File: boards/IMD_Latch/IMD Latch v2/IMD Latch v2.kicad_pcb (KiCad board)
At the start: 2 copper layers, 40 x 35 mm, 17 parts, among them J1 micromatch_female_RA_8, J2 Ultrafit_2, K1 G5Q-1A4-DC5-5V, Q1 SSM3K333R, U1 CD4043BPWR

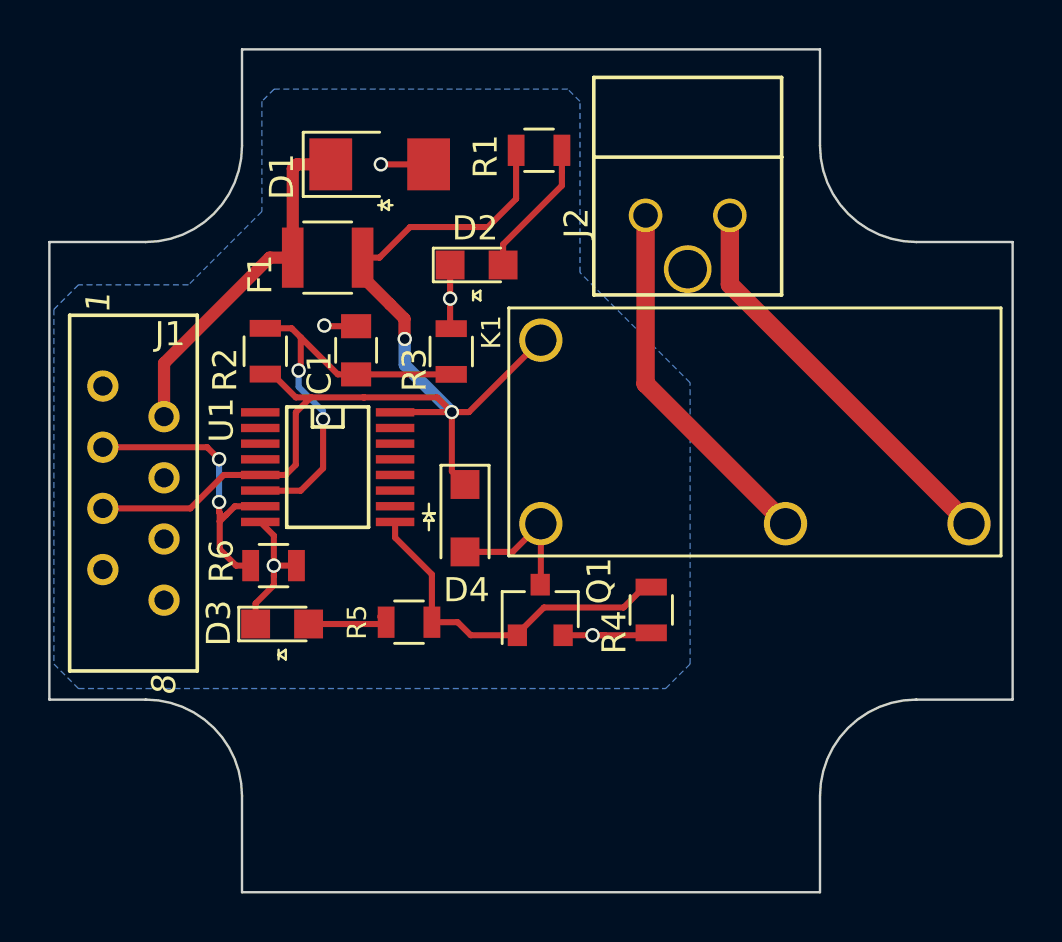
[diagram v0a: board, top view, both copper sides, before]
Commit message: IMD Latch v2 not yet checked off
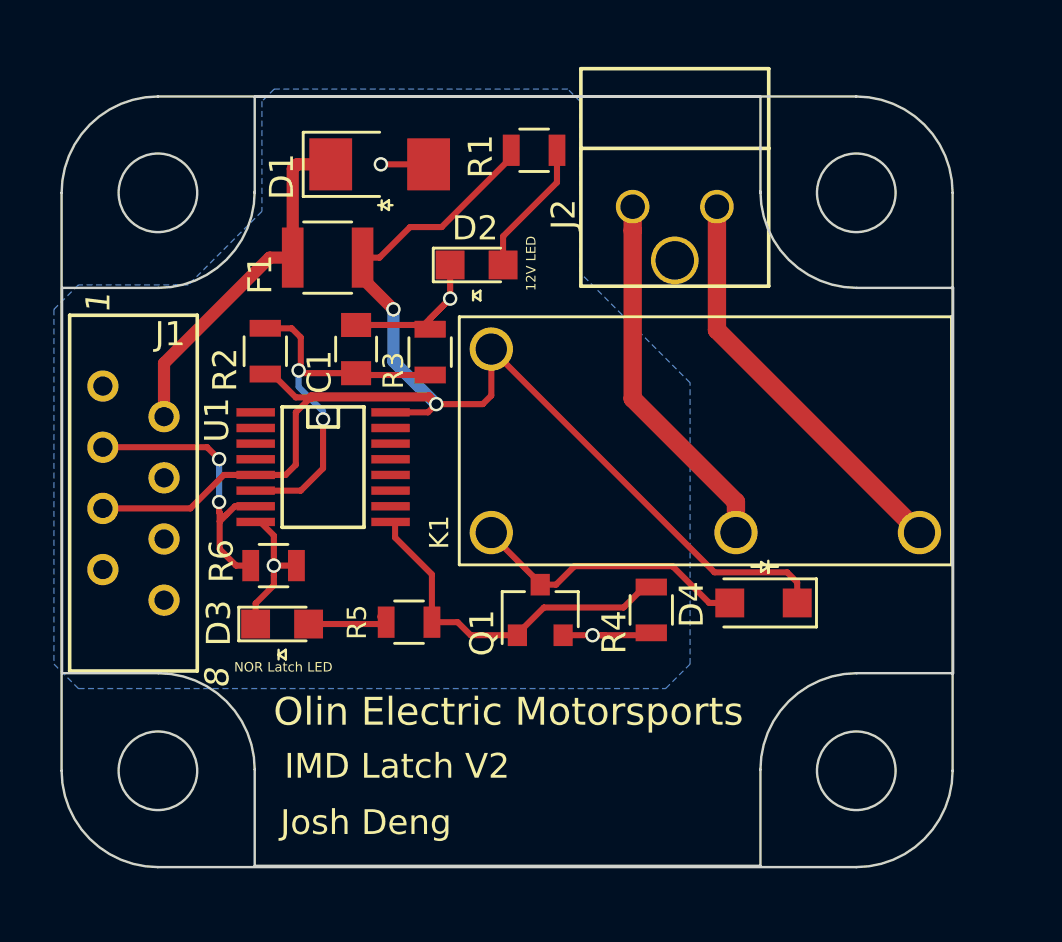
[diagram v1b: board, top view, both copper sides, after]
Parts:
- moved D4 12.9 mm to (169.4, 112.1), turned to 180 degrees
- moved K1 2.09 mm to (158.1, 109.2)
- moved R3 0.88 mm to (155.5, 101.7)
- moved J2 0.65 mm to (167.4, 95.7)
- moved R1 0.20 mm to (159.8, 93.3)
- moved U1 0.19 mm to (151.1, 106.5)
- moved C1 0.05 mm to (152.4, 101.6)
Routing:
- net /12V_Fused: track 48.1 -> 59.8 mm
- net Net-(D4-Pad2): track 6.18 -> 11.9 mm
- net GND: track 15.9 -> 19.5 mm, vias 5 -> 4
- net Net-(C1-Pad1): track 17.4 -> 16.1 mm
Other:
- board size 40 x 35 mm -> 37 x 32 mm
- board text added: "12V LED"
- board text added: "IMD Latch V2"
- board text added: "Josh Deng"
- board text added: "NOR Latch LED"
- board text added: "Olin Electric Motorsports"
